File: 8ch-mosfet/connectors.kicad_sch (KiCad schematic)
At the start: 6 parts, among them J9 I2C

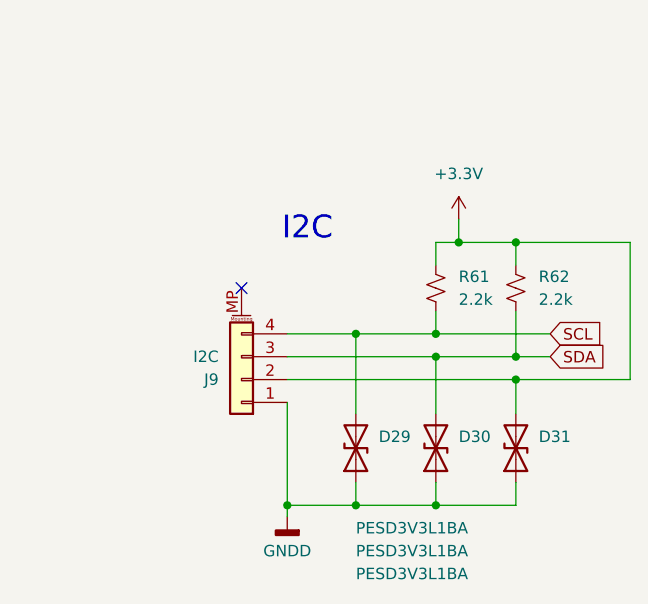
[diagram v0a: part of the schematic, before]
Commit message: component layout looking crispy.
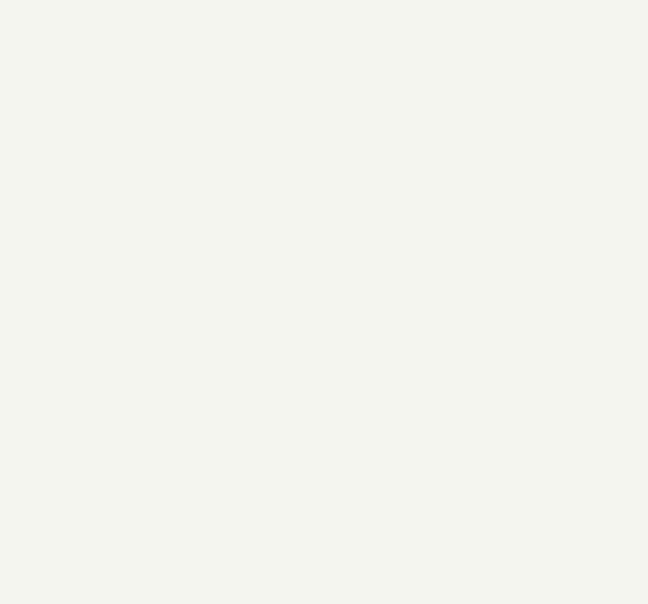
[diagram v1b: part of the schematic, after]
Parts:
- removed D29, D30, D31: PESD3V3L1BA, Diode_SMD:D_SOD-323_HandSoldering, symbol Device:D_TVS
- removed J9: I2C, Connector_JST:JST_SH_SM04B-SRSS-TB_1x04-1MP_P1.00mm_Horizontal, symbol Connector_Generic_MountingPin:Conn_01x04_MountingPin
- removed R61, R62: 2.2k, Resistor_SMD:R_0805_2012Metric_Pad1.20x1.40mm_HandSolder, symbol Device:R_Small_US
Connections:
- no-connect marks 1 -> 0
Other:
- note removed: "I2C"
